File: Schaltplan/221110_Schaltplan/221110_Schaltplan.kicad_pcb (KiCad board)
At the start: 2 copper layers, 27 parts, among them J0 LDR0, J1 LDR1, J10 LDR2, J11 LDR3, J12 V_solar, J13 V_solar, J14 Dspl GND, J15 Dspl Vcc, J16 Mode Button GND, J17 Poti GND, J18 Mode Button, J19 Poti 5V, J2 LDR2, J20 Poti, J3 LDR3, J4 Dspl SDA, J5 Dspl SCL, J6 Srv0, J7 Srv1, J8 LDR0, J9 LDR1, U0 MCP3008

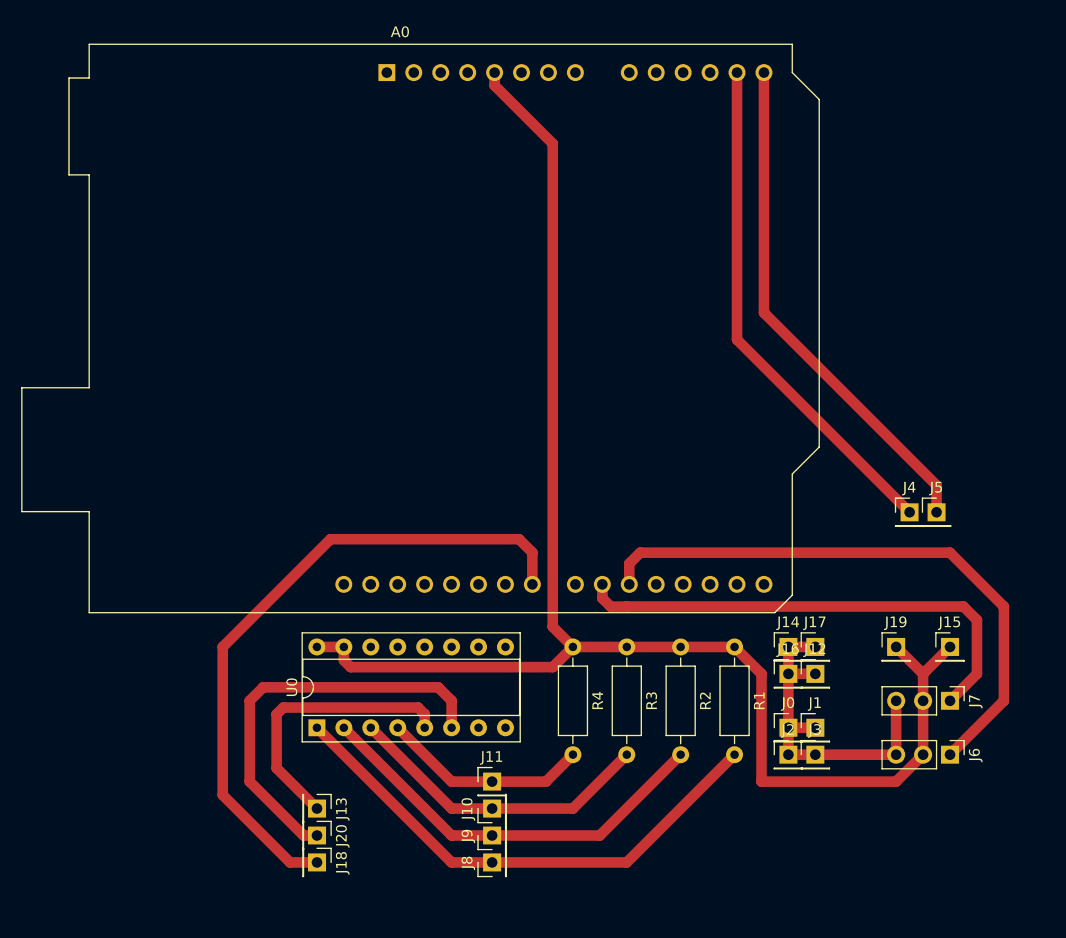
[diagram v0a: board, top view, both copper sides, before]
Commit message: Finish Schaltplan
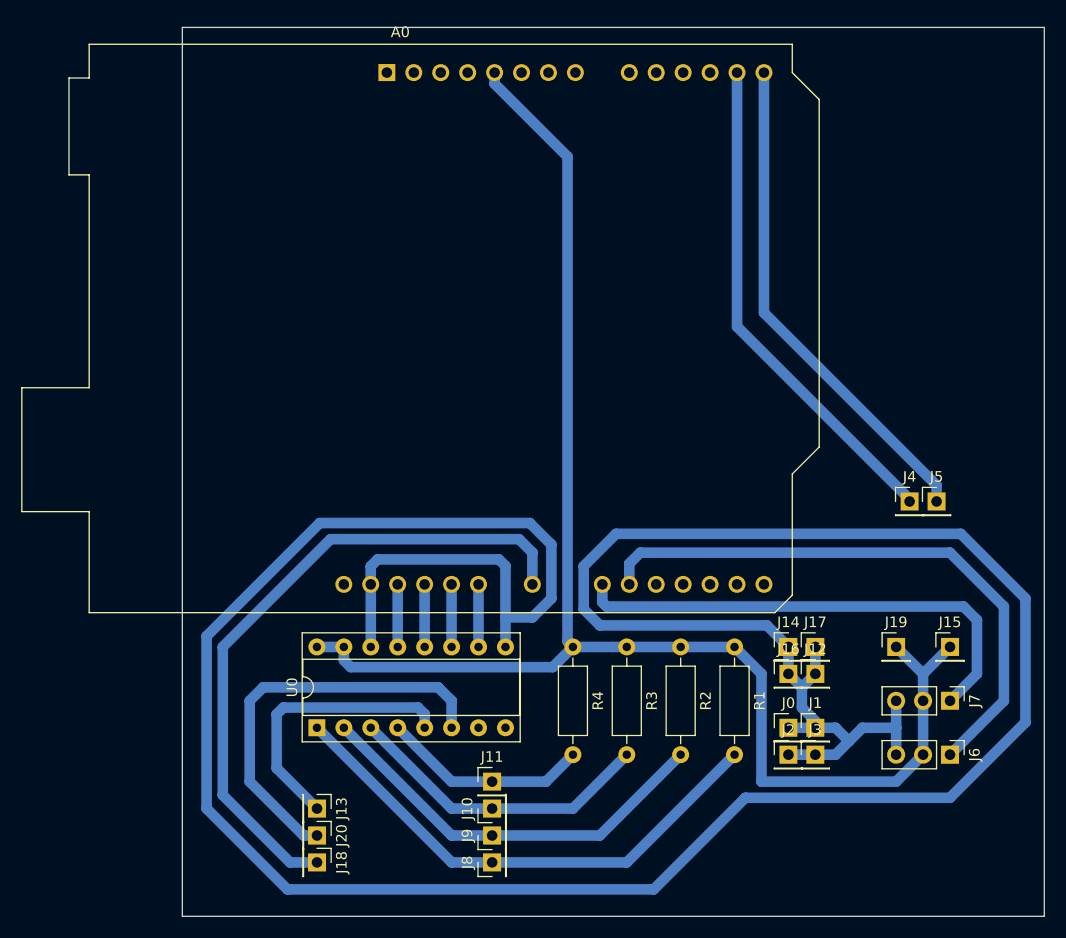
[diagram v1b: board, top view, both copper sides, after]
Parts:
- moved J4 1.02 mm to (174.0, 100.6)
- moved J5 1.02 mm to (176.5, 100.6)
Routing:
- net Net-(A0-Pad29): track 33.0 -> 297.1 mm
- net Net-(A0-Pad26): track 0.00 -> 5.90 mm
- net Net-(A0-Pad28): track 0.00 -> 5.90 mm
- net Net-(A0-Pad27): track 0.00 -> 5.90 mm
- net Net-(A0-Pad25): track 0.00 -> 5.90 mm
- net Net-(A0-Pad14): track 48.2 -> 47.2 mm
- net Net-(A0-Pad13): track 48.2 -> 47.2 mm
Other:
- board outline added: 81.3 x 83.8 mm
